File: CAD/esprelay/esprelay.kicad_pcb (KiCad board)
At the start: 2 copper layers, 65 x 20 mm, 56 parts, among them J1 Conn_01x06_Pin, J2 Conn_01x14_Pin, K1 G6K-2P-Y, K2 G6K-2P-Y, K3 G6K-2P-Y, Q1 Q_Photo_NPN, SW1 SW_SPST, U1 SPX3819M5-L-5-0, U2 SPX3819M5-L-3-3, U3 ESP-12F, U4 SHTC3, U5 TBD62003AFWG

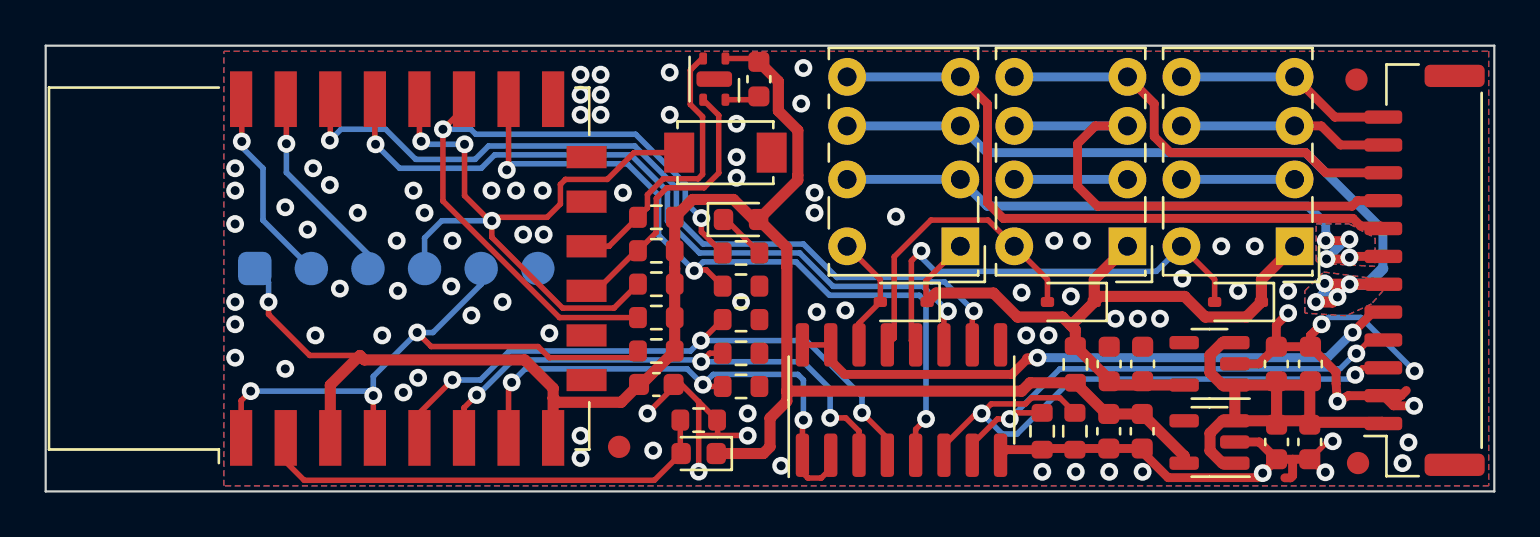
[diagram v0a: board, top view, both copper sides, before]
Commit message: Feat: 4 layer,readme and cleanup
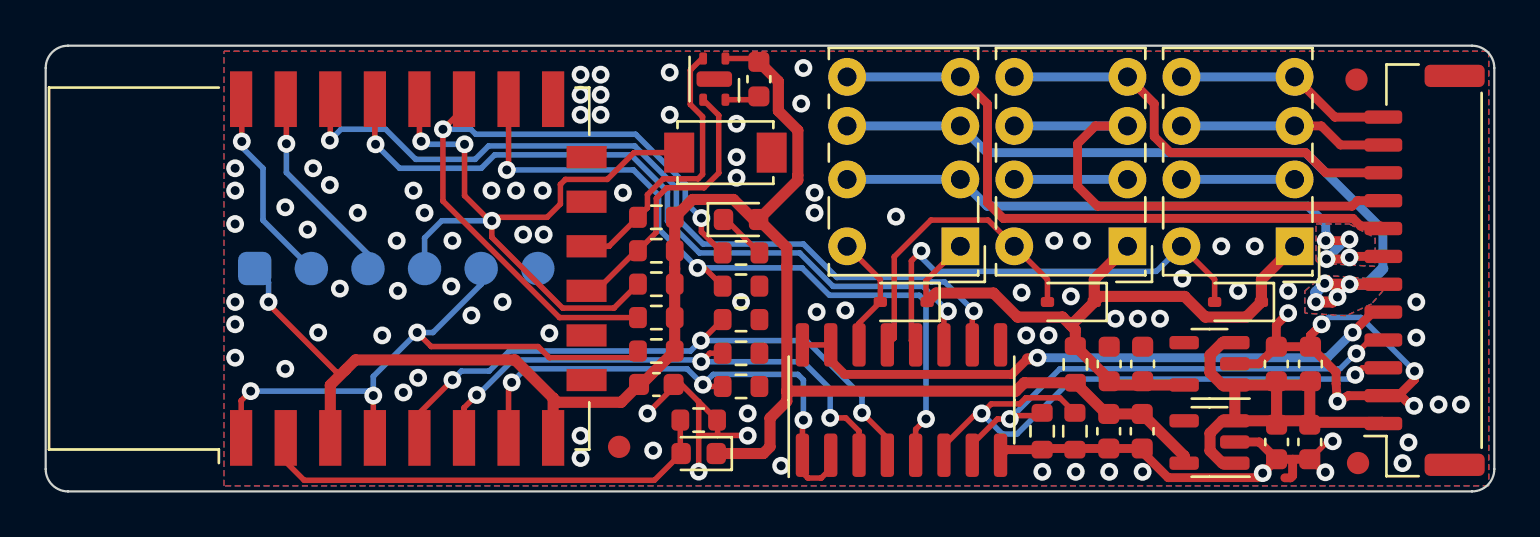
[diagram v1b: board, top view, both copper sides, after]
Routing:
- net GND: track 53.2 -> 54.1 mm, vias 87 -> 91
- net GPIO15: track 34.8 -> 33.9 mm
- net +3.3V: track 83.2 -> 82.7 mm
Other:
- outline, holes or cut-outs redrawn

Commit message: Simplification
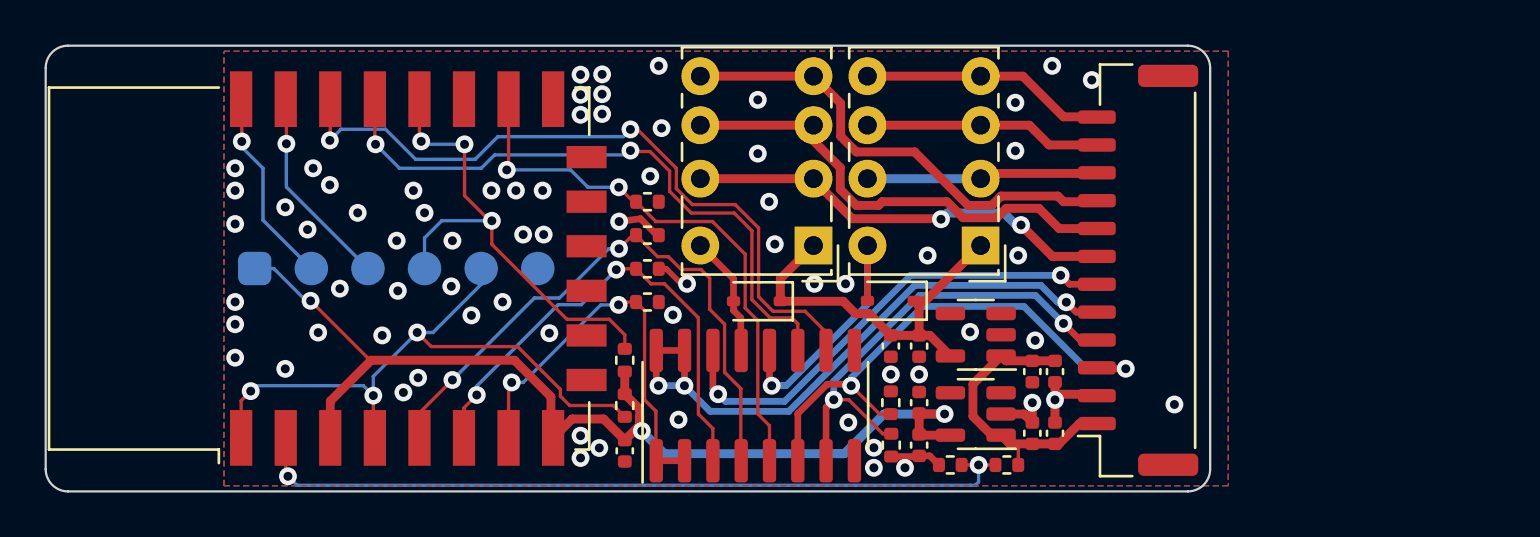
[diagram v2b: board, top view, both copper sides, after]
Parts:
- removed C10: 0.1uF, Capacitor_SMD:C_0603_1608Metric
- removed D3: 1N4148WS, Diode_SMD:D_SOD-323
- removed D4: KT-0603R, LED_SMD:LED_0603_1608Metric
- removed FID1, FID2, FID3: Fiducial, Fiducial:Fiducial_1mm_Mask2mm
- removed JP1: Jumper_2_Open, Resistor_SMD:R_0603_1608Metric
- removed K3: G6K-2P-Y, Relay_THT:Relay_DPDT_Omron_G6K-2P-Y
- removed Q1: Q_Photo_NPN, LED_SMD:LED_0603_1608Metric
- removed R13: 470, Resistor_SMD:R_0603_1608Metric
- removed R4, R5: 10K, Resistor_SMD:R_0603_1608Metric
- removed SW1: SW_SPST, Button_Switch_SMD:SW_SPST_TS-1088-AR
- removed U4: SHTC3, Sensor_Humidity:Sensirion_DFN-4-1EP_2x2mm_P1mm_EP0.7x1.6mm
- removed kibuzzard-65666CB0: G***, kibuzzard-65666CB0
- removed kibuzzard-65666CF7: G***, kibuzzard-65666CF7
- removed kibuzzard-65666CFD: G***, kibuzzard-65666CFD
- removed kibuzzard-65666D06: G***, kibuzzard-65666D06
- removed kibuzzard-65666D10: G***, kibuzzard-65666D10
- removed kibuzzard-65666D19: G***, kibuzzard-65666D19
- added kibuzzard-65CFDA91: G***, kibuzzard-65CFDA91, B.Cu at (149.1, 83.3)
- added kibuzzard-65CFDAA0: G***, kibuzzard-65CFDAA0, B.Cu at (149.1, 80.2)
- added kibuzzard-65CFDAA7: G***, kibuzzard-65CFDAA7, B.Cu at (149.1, 78.7)
- added kibuzzard-65CFDAAD: G***, kibuzzard-65CFDAAD, B.Cu at (149.1, 77.1)
- added kibuzzard-65CFDAB5: G***, kibuzzard-65CFDAB5, B.Cu at (149.1, 75.6)
- added kibuzzard-65CFDABC: G***, kibuzzard-65CFDABC, B.Cu at (149.1, 74.0)
- C1, C2, C6, C7: value 22uF -> 2.2uF; footprint Capacitor_SMD:C_0603_1608Metric -> Capacitor_SMD:C_0402_1005Metric
- C3, C4, C5, C8, C9: footprint Capacitor_SMD:C_0603_1608Metric -> Capacitor_SMD:C_0402_1005Metric
- J2: value Conn_01x14_Pin -> SM12B-GHS-TB(LF)(SN)
- R1, R10, R11, R12, R2, R7, R8, R9: footprint Resistor_SMD:R_0603_1608Metric -> Resistor_SMD:R_0402_1005Metric
- R3: value 10K -> 137k; footprint Resistor_SMD:R_0603_1608Metric -> Resistor_SMD:R_0402_1005Metric
- R6: value 470 -> 316k; footprint Resistor_SMD:R_0603_1608Metric -> Resistor_SMD:R_0402_1005Metric
- U1: value SPX3819M5-L-5-0 -> DS8242-33S5
- U2: value SPX3819M5-L-3-3 -> DS8242-50S3
- moved R3 14.8 mm to (140.6, 91.3), turned to 180 degrees
- moved R6 14.0 mm to (143.1, 91.3), turned to 180 degrees
- moved kibuzzard-65666C7B 13.0 mm to (149.1, 86.4)
- moved kibuzzard-65666C6B 13.0 mm to (149.1, 91.1)
- moved kibuzzard-65666C71 13.0 mm to (149.1, 89.5)
- moved kibuzzard-65666C76 13.0 mm to (149.1, 88.0)
- moved kibuzzard-65666C87 13.0 mm to (149.1, 84.9)
- moved kibuzzard-65666CB7 13.0 mm to (149.1, 81.8)
- moved J2 12.9 mm to (149.0, 82.6)
- moved C5 12.5 mm to (144.3, 87.1), turned to 90 degrees
- moved U2 11.5 mm to (141.7, 85.5)
- moved C1 11.4 mm to (145.3, 89.9), turned to 90 degrees
- moved C8 11.3 mm to (137.9, 86.0), turned to -90 degrees
- moved C4 11.0 mm to (144.3, 89.9), turned to -90 degrees
- moved U1 10.7 mm to (141.7, 89.0)
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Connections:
- J2 pad 10: R2NO -> R2NC
- J2 pad 11: R3A -> R2CO
- J2 pad 12: R3NO -> R2NO
- J2 pad 6: R1A -> HO2
- J2 pad 8: R1NO -> R1CO
- J2 pad 9: R2A -> R1NO
- K1 pad 3: R1A -> R1CO
- K1 pad 6: R1A -> R1CO
- K2 pad 3: R2A -> R2CO
- K2 pad 6: R2A -> R2CO
- R3 pad 1: GPIO2 -> ADC
- R3 pad 2: +3.3V -> GND
- R6 pad 1: PHOTO_OUT -> +VDC
- R6 pad 2: GND -> ADC
- U1 pad 3: +VDC -> unconnected-(U1-NC-Pad3)
- U1 pad 5: VBUS -> +3.3V
- U2 pad 3: +VDC -> unconnected-(U2-NC-Pad3)
- U2 pad 5: +3.3V -> VBUS
- U3 pad 11: SDA -> unconnected-(U3-GPIO9-Pad11)
- U3 pad 12: SCL -> unconnected-(U3-GPIO10-Pad12)
- U3 pad 17: GPIO2 -> unconnected-(U3-GPIO2-Pad17)
- U3 pad 2: PHOTO_OUT -> ADC
- U5 pad 12: RO3 -> RO2
- U5 pad 13: RO2 -> RO1
- U5 pad 14: RO1 -> HO2
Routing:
- net GND: track 54.1 -> 12.3 mm, vias 91 -> 70
- net ADC: track 0.00 -> 35.3 mm, vias 0 -> 2
- net R1A: track 34.2 -> 0.00 mm, vias 4 -> 0
- net +3.3V: track 82.7 -> 48.8 mm, vias 1 -> 3
- net GPIO2: track 31.6 -> 0.00 mm, vias 2 -> 0
- net R2A: track 23.7 -> 0.00 mm
- net HO2: track 0.00 -> 21.7 mm, vias 0 -> 2
- net R1CO: track 0.00 -> 21.2 mm
- net PHOTO_OUT: track 21.2 -> 0.00 mm
- net RO3: track 20.3 -> 0.00 mm, vias 1 -> 0
- net VBUS: track 33.0 -> 17.4 mm
- net SDA: track 12.6 -> 0.00 mm
- net SCL: track 12.6 -> 0.00 mm
- net R2CO: track 0.00 -> 10.7 mm
- net BOOT: track 32.3 -> 22.0 mm
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- removed copper zone on B.Cu, net R1A
- removed copper zone on F.Cu, net R1A
- removed copper zone on B.Cu, net R1NC
- removed copper zone on F.Cu, net R1NC
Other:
- board size 65 x 20 mm -> 52.2 x 20 mm
